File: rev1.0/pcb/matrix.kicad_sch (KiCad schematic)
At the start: 103 parts

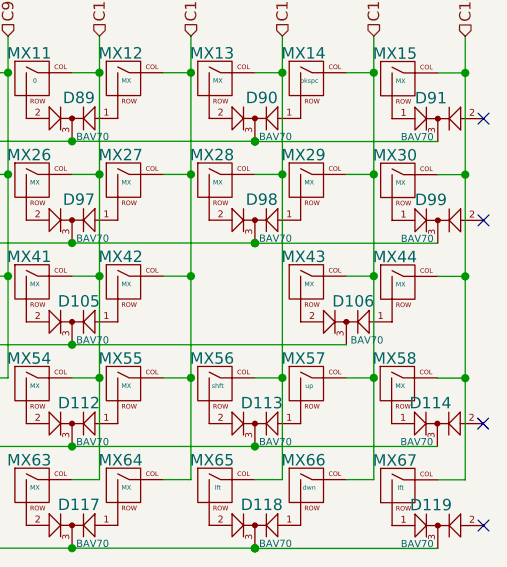
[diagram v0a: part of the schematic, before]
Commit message: Did the rows... again
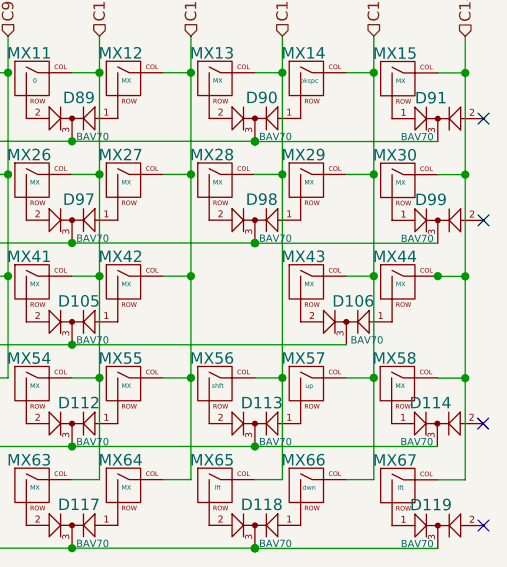
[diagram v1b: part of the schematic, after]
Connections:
- net C14: no longer MX44.1 (COL)
- net at MX44.2 (ROW): now also D106.1 (A1)
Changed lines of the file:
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@@
   (junction (at 176.276 58.547) (diameter 0) (color 0 0 0 0))
   (junction (at 176.276 69.85) (diameter 0) (color 0 0 0 0))
+  (junction (at 183.388 58.547) (diameter 0) (color 0 0 0 0))
   (junction (at 186.436 35.9664) (diameter 0) (color 0 0 0 0))
   (junction (at 186.436 47.2694) (diameter 0) (color 0 0 0 0))
@@
     (pin "2")
   )
-  (symbol (lib_id "0xcb:MX") (at 179.578 58.5724 0) (unit 1)
-    (in_bom yes) (on_board yes)
-    (property "Reference" "MX44" (id 0) (at 178.6255 56.4134 0))
-    (property "Value" "MX" (id 1) (at 179.2605 59.4614 0)
-      (effects (font (size 0.508 0.508)))
-    )
-    (property "Footprint" "0xcb:SW_Hotswap_Kailh_1.00u" (id 2) (at 180.848 56.0324 0)
-      (effects (font (size 1.27 1.27)) hide)
-    )
-    (property "Datasheet" "" (id 3) (at 180.848 56.0324 0)
-      (effects (font (size 1.27 1.27)) hide)
-    )
+  (symbol (lib_id "0xcb:MX") (at 179.578 58.547 0) (unit 1)
+    (in_bom yes) (on_board yes)
+    (property "Reference" "MX44" (id 0) (at 178.6255 56.388 0))
+    (property "Value" "MX" (id 1) (at 179.2605 59.436 0)
+      (effects (font (size 0.508 0.508)))
+    )
+    (property "Footprint" "0xcb:SW_Hotswap_Kailh_1.00u" (id 2) (at 180.848 56.007 0)
+      (effects (font (size 1.27 1.27)) hide)
+    )
+    (property "Datasheet" "" (id 3) (at 180.848 56.007 0)
+      (effects (font (size 1.27 1.27)) hide)
+    )

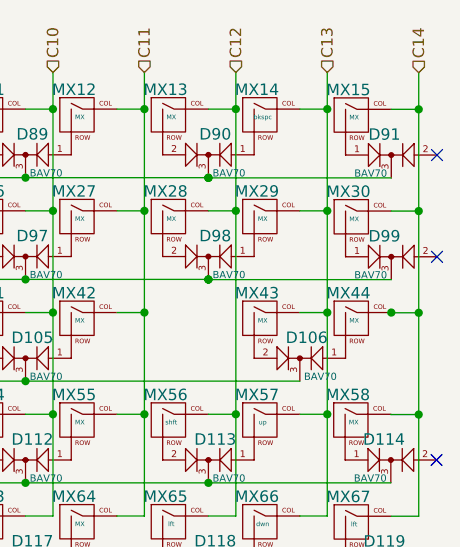
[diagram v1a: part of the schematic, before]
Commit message: RGB LED Stuff
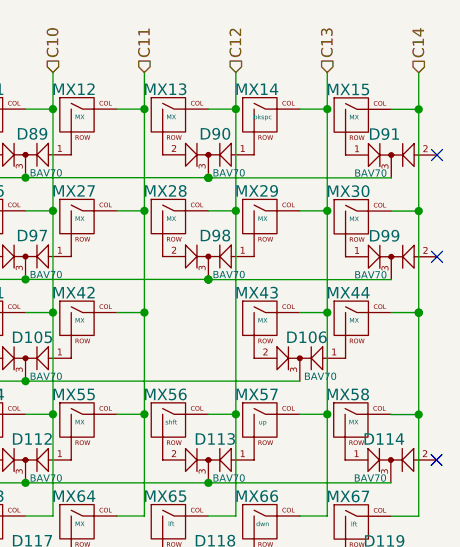
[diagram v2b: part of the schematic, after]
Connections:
- net C14: now also MX44.1 (COL)
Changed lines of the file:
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@@
   (junction (at 176.276 58.547) (diameter 0) (color 0 0 0 0))
   (junction (at 176.276 69.85) (diameter 0) (color 0 0 0 0))
-  (junction (at 183.388 58.547) (diameter 0) (color 0 0 0 0))
   (junction (at 186.436 35.9664) (diameter 0) (color 0 0 0 0))
   (junction (at 186.436 47.2694) (diameter 0) (color 0 0 0 0))
+  (junction (at 186.436 58.547) (diameter 0) (color 0 0 0 0))
   (junction (at 186.436 58.5709) (diameter 0) (color 0 0 0 0))
   (junction (at 186.436 69.8794) (diameter 0) (color 0 0 0 0))
@@
     (stroke (width 0) (type default) (color 0 0 0 0))
   )
-  (wire (pts (xy 183.388 58.5709) (xy 183.388 58.5724))
-    (stroke (width 0) (type default) (color 0 0 0 0))
-  )
   (wire (pts (xy 183.388 88.7984) (xy 163.068 88.7984))
     (stroke (width 0) (type default) (color 0 0 0 0))
@@
     (stroke (width 0) (type solid) (color 0 0 0 0))
   )
-  (wire (pts (xy 186.436 47.2694) (xy 186.436 58.5709))
-    (stroke (width 0) (type default) (color 0 0 0 0))
-  )
-  (wire (pts (xy 186.436 58.5709) (xy 183.388 58.5709))
-    (stroke (width 0) (type default) (color 0 0 0 0))
-  )
+  (wire (pts (xy 186.436 47.2694) (xy 186.436 58.547))
+    (stroke (width 0) (type default) (color 0 0 0 0))
+  )
+  (wire (pts (xy 186.436 58.547) (xy 183.388 58.547))
+    (stroke (width 0) (type default) (color 0 0 0 0))
+  )
+  (wire (pts (xy 186.436 58.547) (xy 186.436 58.5709))
+    (stroke (width 0) (type default) (color 0 0 0 0))
+  )
